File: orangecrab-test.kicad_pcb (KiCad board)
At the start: 2 copper layers, 156.4 x 77.5 mm, 156 parts, among them J1 Conn_01x16, J2 Conn_01x12, J3 USB_B_Micro, J4 JTAG, Q1 DMG2302UK-7, SW1 SW_Push, U1 DAC53608RTET, U2 MCP23S08T-E-ML, U3 93C46B/SN, U4 FT232HL-REEL, U5 TPS76301DBVR, Y1 12MHz

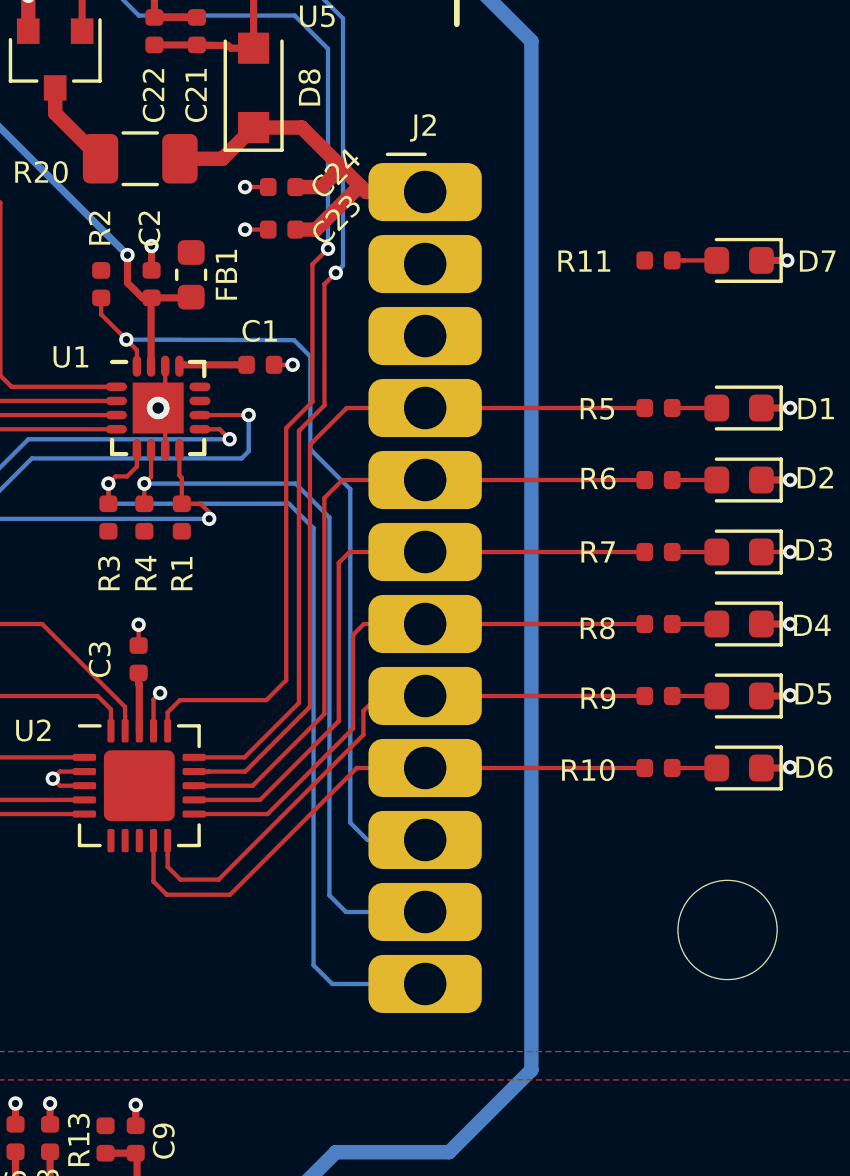
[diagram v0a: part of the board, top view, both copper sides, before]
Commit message: r0.0 release:  - Design review  - Fixed minor error  - Validate BOM  - Generate and package gerbers for fabrication
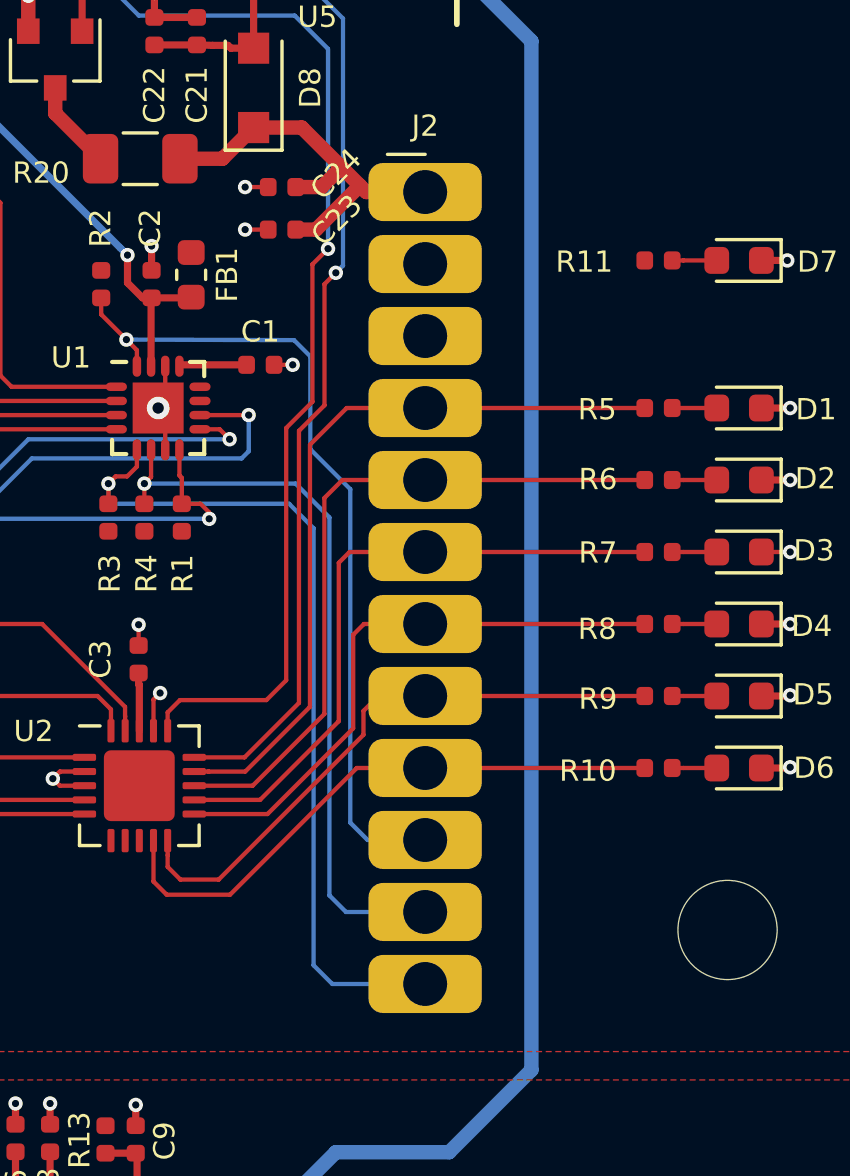
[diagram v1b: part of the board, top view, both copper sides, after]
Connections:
- C15 pad 1: Net-(C15-Pad1) -> +3.3VA
- U3 pad 8: Net-(C15-Pad1) -> +3.3VA
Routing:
- net +3.3VA: track 11.5 -> 13.2 mm
- net Net-(C15-Pad1): track 1.68 -> 0.00 mm
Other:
- rule solder_mask_min_width: 0.25 -> 0.02
